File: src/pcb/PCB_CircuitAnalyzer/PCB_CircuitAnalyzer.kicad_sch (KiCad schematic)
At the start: 1 part, among them U1 74AHC240

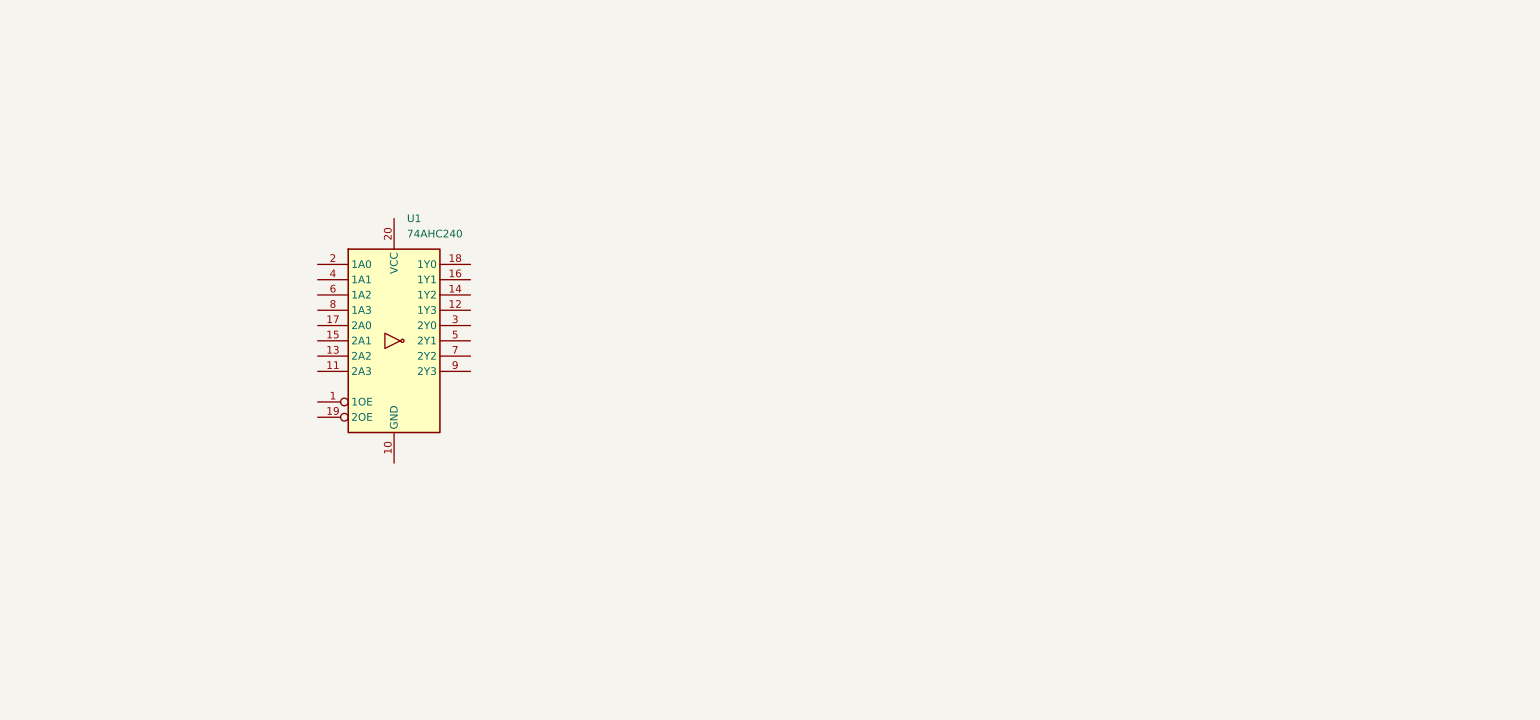
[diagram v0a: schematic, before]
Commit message: finished schematic
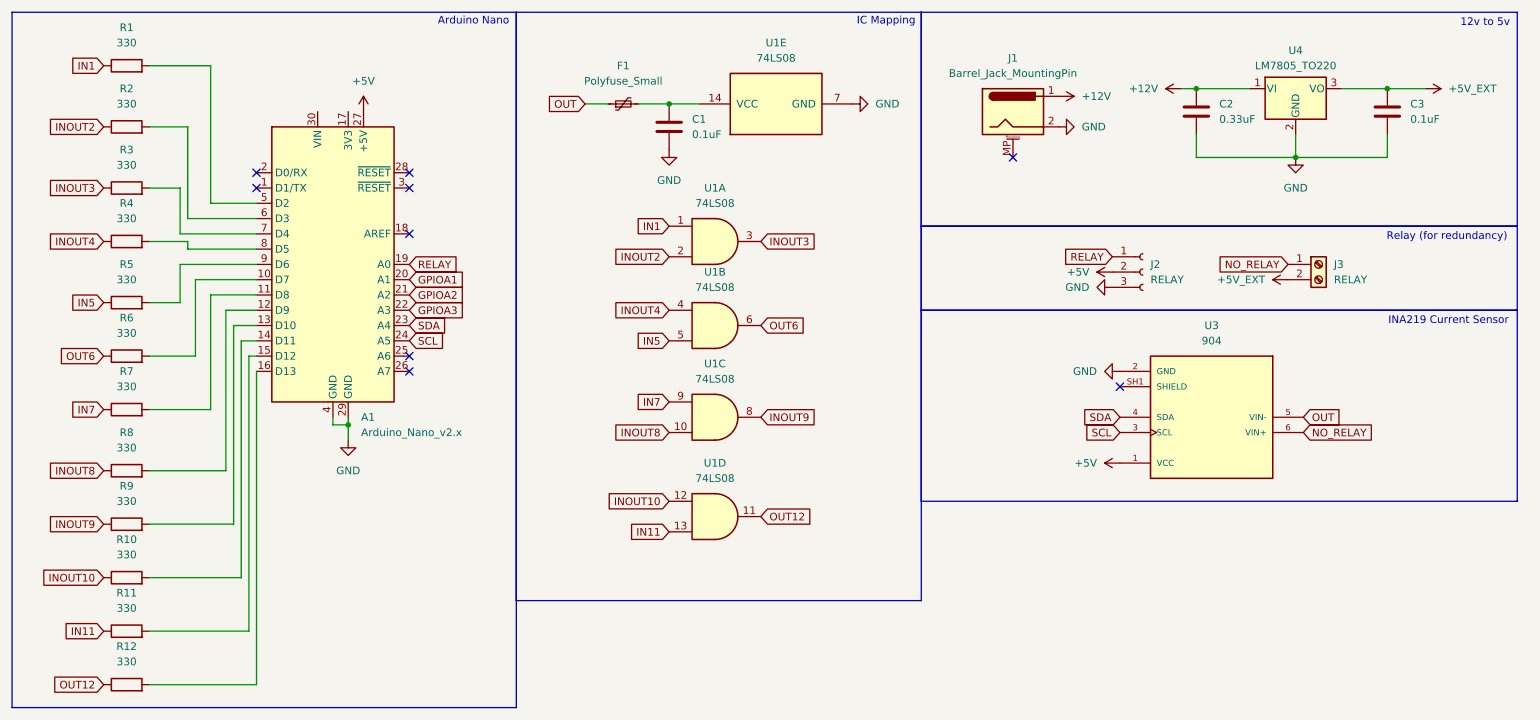
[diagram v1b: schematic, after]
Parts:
- removed U1: 74AHC240, symbol 74xx:74AHC240
- added A1: Arduino_Nano_v2.x, Module:Arduino_Nano, symbol MCU_Module:Arduino_Nano_v2.x
- added C1, C3: 0.1uF, Capacitor_THT:C_Axial_L3.8mm_D2.6mm_P7.50mm_Horizontal, symbol Device:C
- added C2: 0.33uF, Capacitor_THT:C_Axial_L3.8mm_D2.6mm_P7.50mm_Horizontal, symbol Device:C
- added F1: Polyfuse_Small, Capacitor_THT:C_Axial_L3.8mm_D2.6mm_P7.50mm_Horizontal, symbol Device:Polyfuse_Small
- added J1: Barrel_Jack_MountingPin, Connector_BarrelJack:BarrelJack_GCT_DCJ200-10-A_Horizontal, symbol Connector:Barrel_Jack_MountingPin
- added J2: RELAY, Connector_PinSocket_2.54mm:PinSocket_1x03_P2.54mm_Vertical, symbol Connector:Conn_01x03_Socket
- added J3: RELAY, TerminalBlock_Phoenix:TerminalBlock_Phoenix_MKDS-1,5-2_1x02_P5.00mm_Horizontal, symbol Connector:Screw_Terminal_01x02
- added R1, R10, R11, R12, R2, R3, R4, R5, R6, R7, R8, R9: 330, Resistor_THT:R_Axial_DIN0204_L3.6mm_D1.6mm_P5.08mm_Horizontal, symbol Device:R
- added U1: 74LS08, Socket:DIP_Socket-14_W4.3_W5.08_W7.62_W10.16_W10.9_3M_214-3339-00-0602J, symbol 74xx:74LS08
- added U3: 904, Snapeda:MODULE_904, symbol Snapeda:904
- added U4: LM7805_TO220, Package_TO_SOT_THT:TO-220-3_Horizontal_TabDown, symbol Regulator_Linear:LM7805_TO220
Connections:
- new net: A1.6 (D3), R2.2
- new net: A1.14 (D11), R10.2
- new net: A1.8 (D5), R4.2
- new net: A1.9 (D6), R5.2
- new net: A1.13 (D10), R9.2
- new net: C1.1, F1.2, U1.14 (VCC)
- new net: A1.15 (D12), R11.2
- new net: A1.12 (D9), R8.2
- new net: A1.10 (D7), R6.2
- new net: A1.11 (D8), R7.2
- new net: A1.16 (D13), R12.2
- new net: A1.5 (D2), R1.2
- new net: A1.7 (D4), R3.2
- new net: U3.SH1 (SHIELD), U3.SH2 (SHIELD), U3.SH3 (SHIELD), U3.SH4 (SHIELD)
- new net +12V: C2.1, J1.1, U4.1 (VI)
- new net +5V: A1.27 (+5V), J2.2 (Pin_2), U3.1 (VCC)
- new net +5V_EXT: C3.1, J3.2 (Pin_2), U4.3 (VO)
- new net GND: A1.29 (GND), A1.4 (GND), C1.2, C2.2, C3.2, J1.2, J2.3 (Pin_3), U1.7 (GND), U3.2 (GND), U4.2 (GND)
- new net GPIOA1: A1.20 (A1)
- new net GPIOA2: A1.21 (A2)
- new net GPIOA3: A1.22 (A3)
- new net IN1: R1.1, U1.1
- new net IN11: R11.1, U1.13
- new net IN5: R5.1, U1.5
- new net IN7: R7.1, U1.9
- new net INOUT10: R10.1, U1.12
- new net INOUT2: R2.1, U1.2
- new net INOUT3: R3.1, U1.3
- new net INOUT4: R4.1, U1.4
- new net INOUT8: R8.1, U1.10
- new net INOUT9: R9.1, U1.8
- new net NO_RELAY: J3.1 (Pin_1), U3.6 (VIN+), U3.VIN+
- new net OUT: F1.1, U3.5 (VIN-), U3.VIN-
- new net OUT12: R12.1, U1.11
- new net OUT6: R6.1, U1.6
- new net RELAY: A1.19 (A0), J2.1 (Pin_1)
- new net SCL: A1.24 (A5), U3.3 (SCL)
- new net SDA: A1.23 (A4), U3.4 (SDA)
- no-connect marks 0 -> 9
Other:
- note added: "12v to 5v"
- note added: "Arduino Nano"
- note added: "IC Mapping"
- note added: "INA219 Current Sensor"
- note added: "Relay (for redundancy)"
